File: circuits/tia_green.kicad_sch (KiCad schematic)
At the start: 11 parts, among them U3 OPA380AID

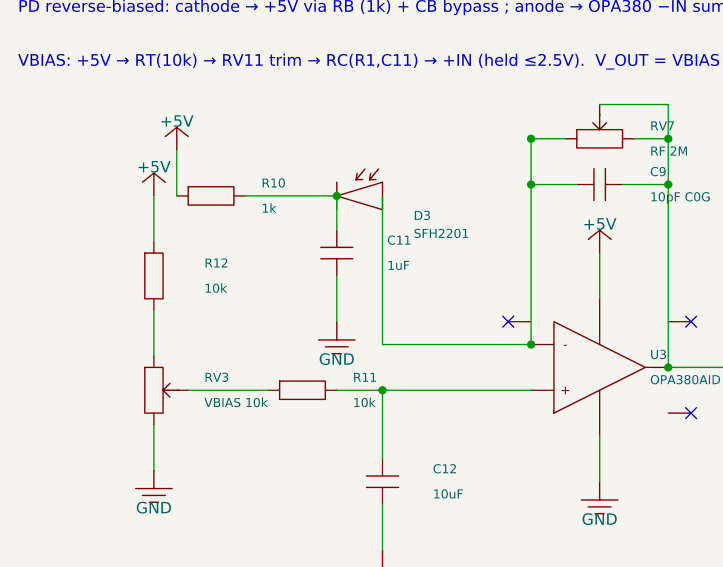
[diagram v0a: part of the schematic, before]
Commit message: Checkpoint laser controller fab parity package
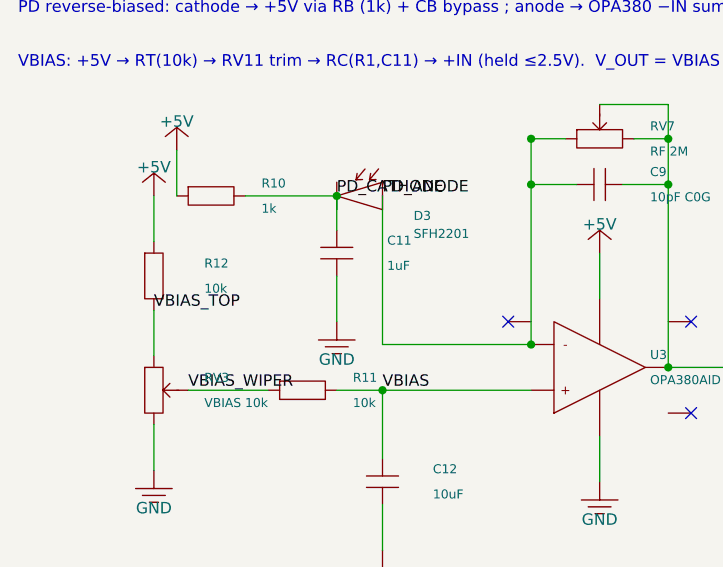
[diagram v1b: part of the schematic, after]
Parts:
- removed C9: 10pF C0G, Capacitor_SMD:C_0603_1608Metric_Pad1.08x0.95mm_HandSolder, symbol viv:C_H
- removed R12: 10k, Resistor_SMD:R_0603_1608Metric_Pad0.98x0.95mm_HandSolder, symbol viv:R_V
- removed RV7: RF 2M, Potentiometer_SMD:Potentiometer_Bourns_3224W_Vertical, symbol viv:POT_H
- added C10: 100nF, Capacitor_SMD:C_0402_1005Metric_Pad0.74x0.62mm_HandSolder, symbol viv:C_V
- added C12: 10uF, Capacitor_SMD:C_0805_2012Metric_Pad1.18x1.45mm_HandSolder, symbol viv:C_V
- added R11: 10k, Resistor_SMD:R_0603_1608Metric_Pad0.98x0.95mm_HandSolder, symbol viv:R_H
- C9: renamed from R11; value 10k -> 10pF C0G; footprint Resistor_SMD:R_0603_1608Metric_Pad0.98x0.95mm_HandSolder -> Capacitor_SMD:C_0603_1608Metric_Pad1.08x0.95mm_HandSolder; symbol viv:R_H -> viv:C_H; LCSC C844918 -> C106245; Part Number CRCW060310K0FKEA -> CC0603JRNPO9BN100
- R12: renamed from C12; value 10uF -> 10k; footprint Capacitor_SMD:C_0805_2012Metric_Pad1.18x1.45mm_HandSolder -> Resistor_SMD:R_0603_1608Metric_Pad0.98x0.95mm_HandSolder; symbol viv:C_V -> viv:R_V; LCSC C318691 -> C844918; Part Number CL21A106KAYNNNG -> CRCW060310K0FKEA
- RV3: renamed from C10; value 100nF -> VBIAS 10k; footprint Capacitor_SMD:C_0402_1005Metric_Pad0.74x0.62mm_HandSolder -> Potentiometer_SMD:Potentiometer_Bourns_3224W_Vertical; symbol viv:C_V -> viv:POT_V; LCSC C83056 -> C81348; Part Number 0402B104K160CT -> 3224W-1-103E
- RV7: renamed from RV3; value VBIAS 10k -> RF 2M; symbol viv:POT_V -> viv:POT_H; LCSC C81348 -> C116323; Part Number 3224W-1-103E -> 3224W-1-205E
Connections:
- net +5V: now also R12.1, C10.1; no longer RV3.1
- net GND: now also RV3.3, C10.2, C12.2; no longer R12.2, RV3.2, RV7.3
- net V_OUT: now also C9.2, RV7.2 (W), RV7.3
- net PD_CATHODE: now reaches C11.1, D3.1 (K), R10.2
- net PD_ANODE: now reaches D3.2 (A), U3.2 (-)
- net PD_ANODE: now also C9.1, RV7.1
- new net VBIAS: C12.1, R11.2, U3.3 (+)
- new net VBIAS_TOP: R12.2, RV3.1
- new net VBIAS_WIPER: R11.1, RV3.2 (W)
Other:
- moved on the sheet: RV7
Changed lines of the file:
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@@
   (no_connect (at 224.79 154.94))
   (no_connect (at 224.79 144.78))
+  (label "PD_ANODE" (at 190.5 130.81 0) (effects (font (size 1.27 1.27)) (justify left bottom)))
+  (label "PD_CATHODE" (at 185.42 130.81 0) (effects (font (size 1.27 1.27)) (justify left bottom)))
+  (label "VBIAS_TOP" (at 165.1 143.51 0) (effects (font (size 1.27 1.27)) (justify left bottom)))
+  (label "VBIAS_WIPER" (at 168.91 152.4 0) (effects (font (size 1.27 1.27)) (justify left bottom)))
+  (label "VBIAS" (at 190.5 152.4 0) (effects (font (size 1.27 1.27)) (justify left bottom)))
   (hierarchical_label "V_OUT" (shape output) (at 232.41 149.86 0) (effects (font (size 1.27 1.27)) (justify left)))
   (text "TIA Channel  —  on-board SFH2201 signal PD → OPA380AID transimpedance amp  ·  reused 4× (IR / RED / GREEN / BLUE)" (at 150 104 0) (effects (font (size 2.0 2.0)) (justify left)))
